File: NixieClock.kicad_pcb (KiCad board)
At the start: 2 copper layers, 170 x 140 mm, 169 parts, among them J1 Barrel_Jack, Q1 MPSA42, Q10 MPSA42, Q11 MPSA42, Q12 MPSA42, Q13 KSP92BU, Q14 KSP92BU, Q15 MPSA42, Q16 MPSA42, Q17 MPSA42, Q18 MPSA42, Q19 KSP92BU, Q2 MPSA42, Q20 KSP92BU, Q21 MPSA42, Q22 MPSA42, Q23 KSP92BU, Q24 KSP92BU, Q25 KSP2907A, Q26 IRF644, Q3 MPSA42, Q4 MPSA42, Q5 MPSA42, Q6 MPSA42, Q7 MPSA42, Q8 MPSA42, Q9 MPSA42, SW1 PB400EEQX, SW2 SW_Push, SW3 SW_Push, SW4 SW_Push, U1 L7805, U10 74LS160, U11 74LS160, U12 74LS160, U13 74LS160, U14 74LS160, U15 74HC4060, U16 4028, U17 74LS151, U18 74LS151, U19 74LS151, U2 MC34063AP, U20 4028, U21 74LS151, U3 74LS14, U4 74LS109, U5 74LS10, U6 74LS08, U7 74LS393, U8 74LS20, U9 74LS160, Y1 32.768 kHz - 12.5pF

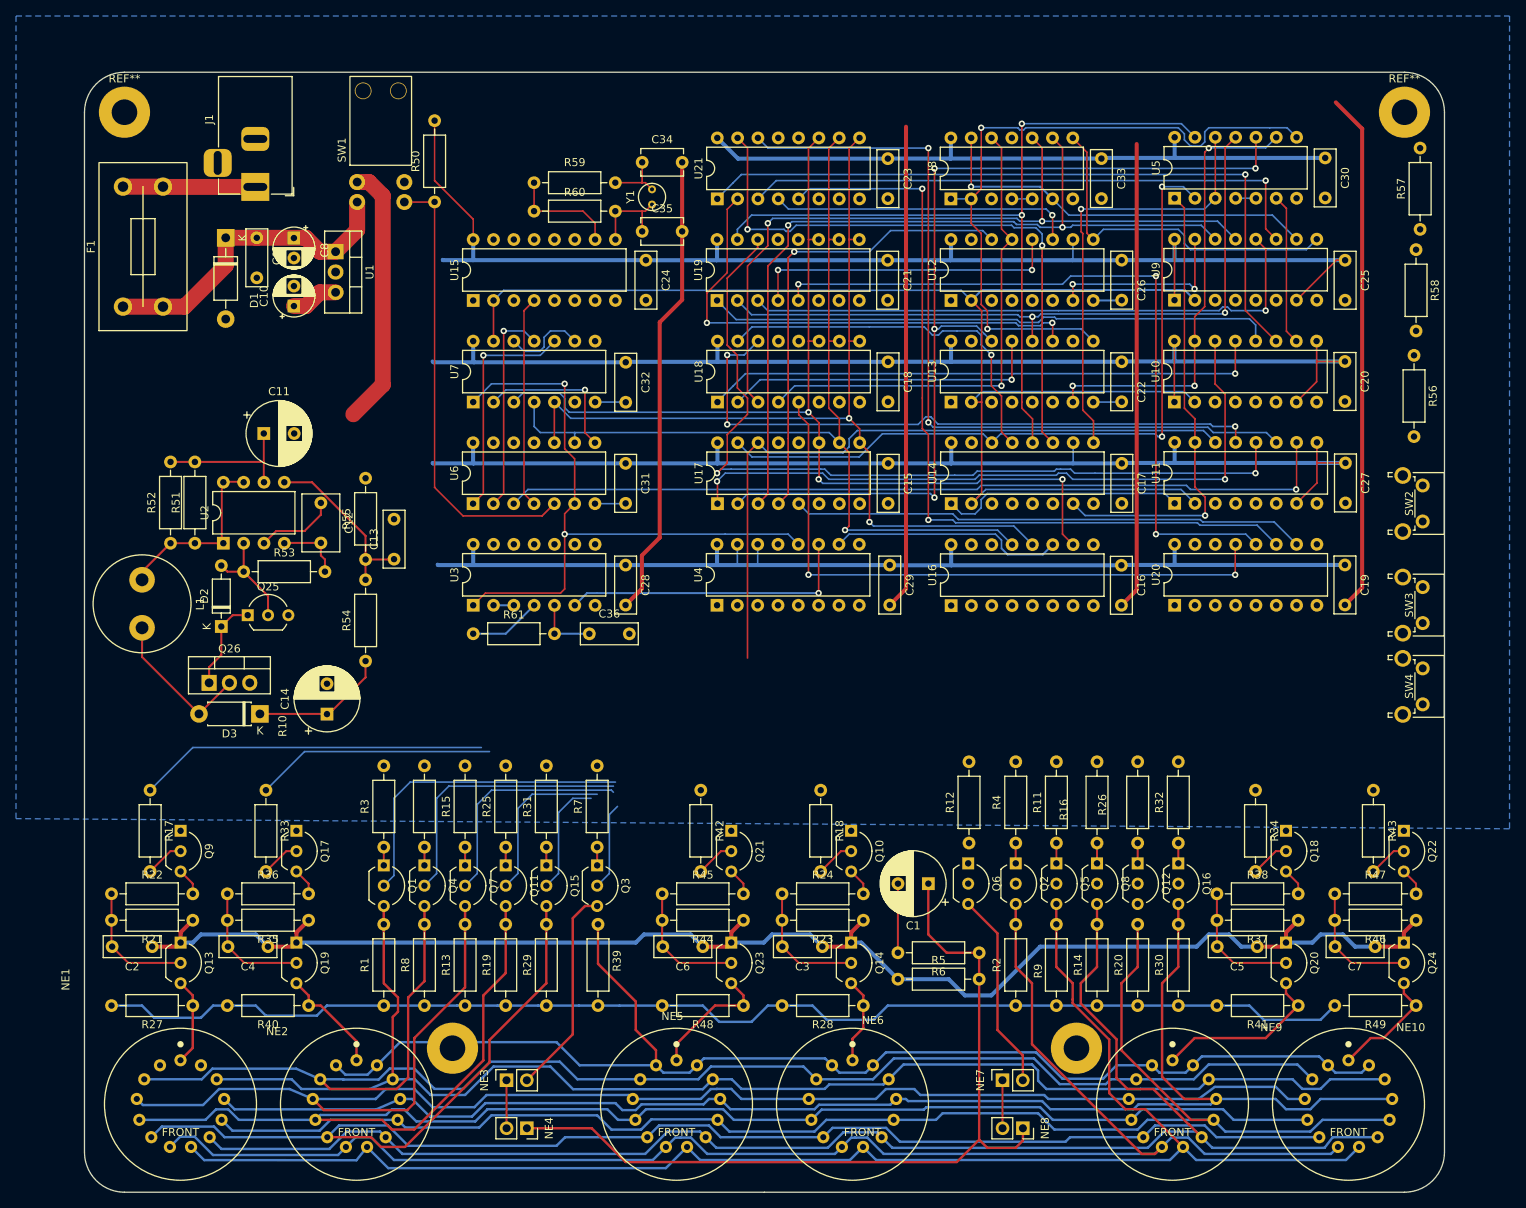
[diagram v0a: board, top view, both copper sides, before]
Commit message: Layout completed
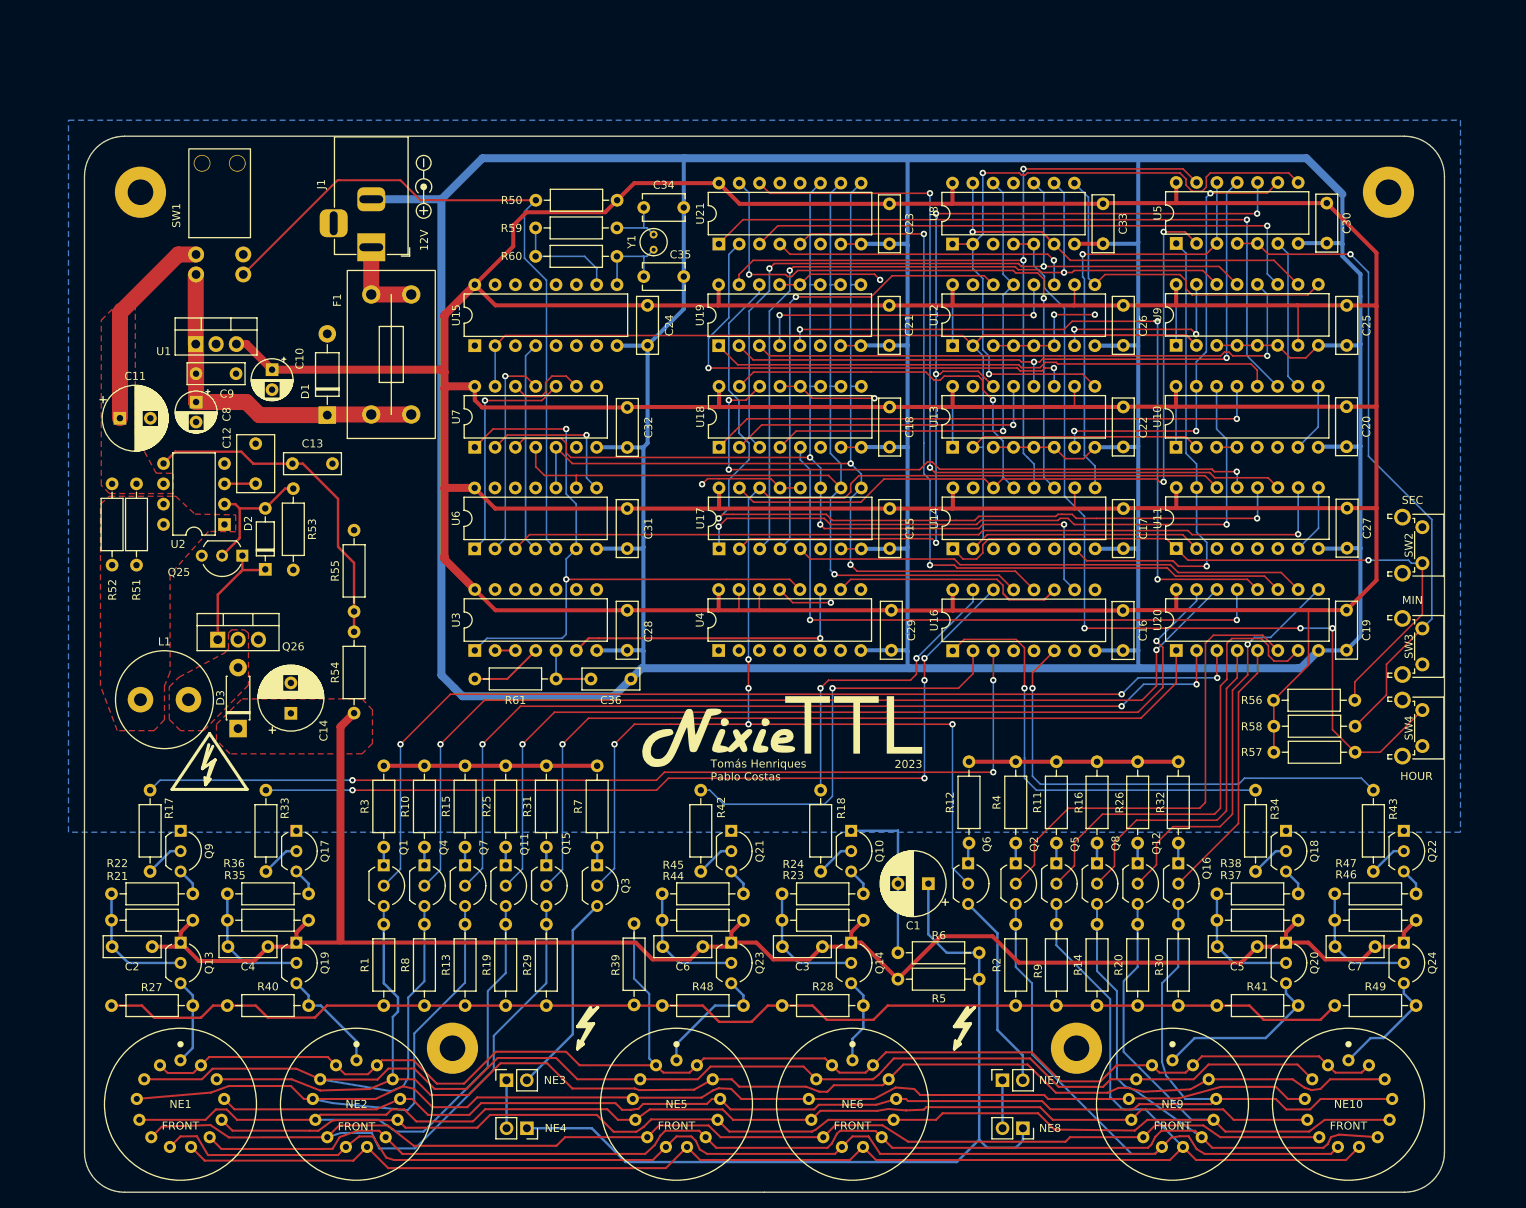
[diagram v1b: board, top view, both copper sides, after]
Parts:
- added 12V: Symbol_Barrel_Polarity, Symbol:Symbol_Barrel_Polarity, F.Cu at (142.5, 35.3)
- added G***: LOGO, NixieClock:NixieTTL_logo, F.Cu at (187.2, 103.2)
- added REF**: Symbol_Highvoltage_Type1_CopperTop_Small, Symbol:Symbol_Highvoltage_Type1_CopperTop_Small, F.Cu at (162.0, 141.1)
- added REF**: Symbol_Highvoltage_Type1_CopperTop_Small, Symbol:Symbol_Highvoltage_Type1_CopperTop_Small, F.Cu at (209.1, 141.1)
- added REF**: Symbol_HighVoltage_Type2_CopperTop_VerySmall, Symbol:Symbol_HighVoltage_Type2_CopperTop_VerySmall, F.Cu at (115.6, 107.9)
- moved R57 67.9 mm to (248.7, 106.0), turned to 0 degrees
- moved R58 62.2 mm to (248.7, 102.8), turned to 0 degrees
- moved R56 46.6 mm to (248.6, 99.5), turned to 0 degrees
- moved F1 33.8 mm to (138.3, 56.3)
- moved D1 25.5 mm to (130.3, 63.9), turned to 90 degrees
- moved C8 23.9 mm to (114.0, 62.2)
- moved SW1 22.1 mm to (119.8, 46.3)
- moved U1 20.9 mm to (113.9, 55.0), turned to 0 degrees
- moved C9 18.6 mm to (114.0, 58.7), turned to 0 degrees
- moved C11 18.1 mm to (104.4, 64.2)
- moved C13 17.4 mm to (126.0, 69.9), turned to 0 degrees
- moved J1 16.3 mm to (135.8, 42.9)
- moved L1 15.0 mm to (107.0, 99.4), turned to 0 degrees
- moved R50 12.7 mm to (156.4, 37.0), turned to 0 degrees
- moved R53 12.1 mm to (126.1, 73.0), turned to -90 degrees
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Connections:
- net Net-(D3-Pad2) renamed /Power Supply/SMPS_SW
- net Net-(L1-Pad1) renamed /Power Supply/SMPS_IN
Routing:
- net GND: track 274.7 -> 833.0 mm, vias 0 -> 6
- net +5V: track 659.9 -> 827.7 mm
- net Net-(R57-Pad2): track 2.54 -> 111.4 mm, vias 0 -> 3
- net CA3: track 20.9 -> 116.2 mm, vias 0 -> 2
- net CA1: track 34.3 -> 126.2 mm, vias 0 -> 2
- net CA4: track 14.6 -> 102.5 mm, vias 0 -> 1
- net CA0: track 40.0 -> 127.5 mm, vias 0 -> 3
- net CA2: track 28.7 -> 115.2 mm, vias 0 -> 3
- net AN2: track 29.9 -> 110.1 mm, vias 0 -> 4
- net Net-(R58-Pad2): track 2.54 -> 81.9 mm, vias 0 -> 1
- net AN1: track 43.6 -> 121.5 mm, vias 0 -> 3
- net S_UN_A: track 98.5 -> 172.8 mm, vias 0 -> 5
- net AN6: track 0.00 -> 60.8 mm, vias 0 -> 1
- net CA5: track 0.00 -> 59.7 mm
- net CA6: track 0.00 -> 58.7 mm
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- added copper zone on F.Cu, net /Power Supply/SMPS_IN
- added copper zone on F.Cu, net /Power Supply/SMPS_SW
- added copper zone on F.Cu, net HT
- added copper zone on F.Cu, net Net-(C11-Pad1)
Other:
- board size 170 x 140 mm -> 170 x 132 mm
- board text added: "2023"
- board text added: "HOUR"
- board text added: "MIN"
- board text added: "SEC"
- board text added: "Tomás Henriques Pablo Costas"
